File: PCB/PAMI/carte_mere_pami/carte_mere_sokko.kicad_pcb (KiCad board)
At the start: 2 copper layers, 78.5 x 54 mm, 35 parts, among them IC1 ESP32-S3-WROOM-1-N16R8, IC2 LDO_3.3V_bis, J1 Conn_01x08_Socket, J10 Conn_01x07_Socket, J11 Conn_01x07_Socket, J12 Conn_Servos, J14 LiDAR Connector, J2 Connector 5V, J3 Connector 3.3V, J4 Micro_USB_pads_USB3075-30-A, J5 Conn_01x08_Socket, J6 Conn_01x04_Pin, J7 Conn_01x04_Pin, J8 Conn_01x08_Socket, J9 Conn_01x08_Socket, U1 ICM-45686

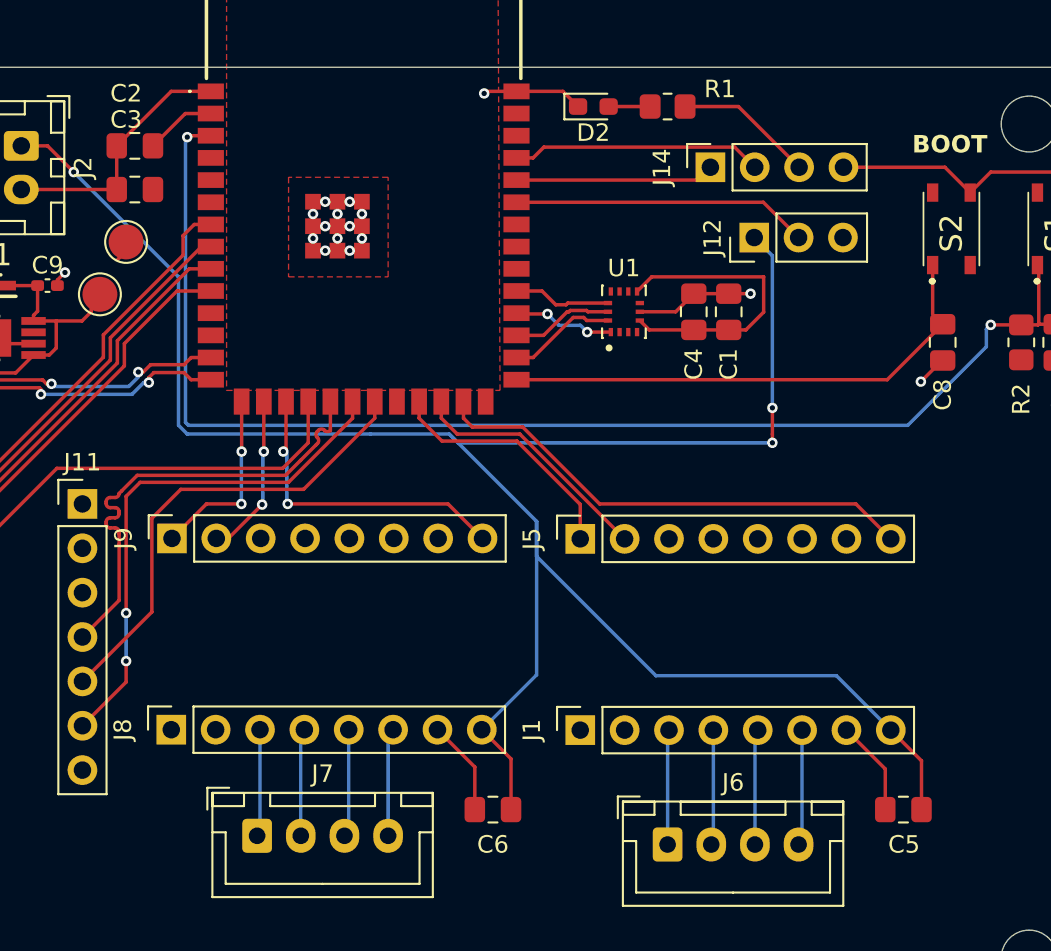
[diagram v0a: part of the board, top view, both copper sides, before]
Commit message: Update hole position
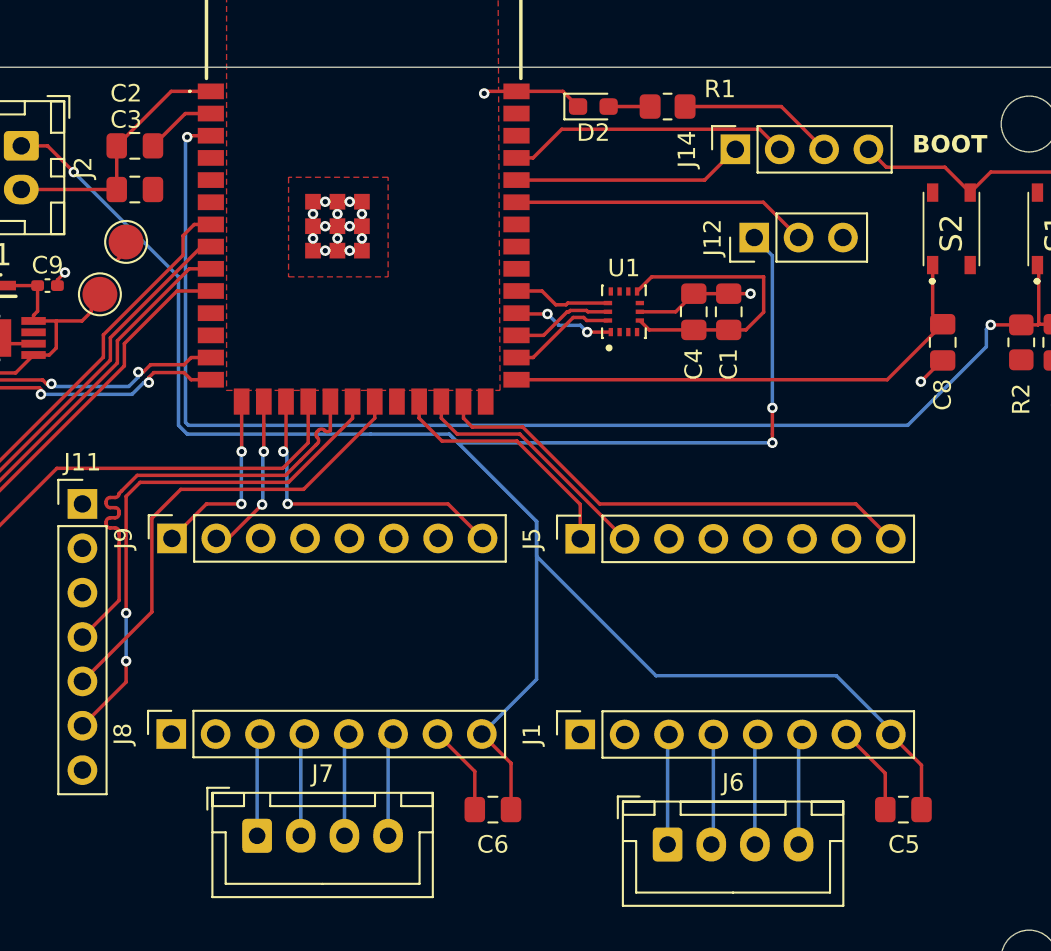
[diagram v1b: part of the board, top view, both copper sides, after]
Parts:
- moved J14 1.76 mm to (184.9, 72.7)
- moved J1 0.25 mm to (176.0, 106.2)
- moved J8 0.25 mm to (152.6, 106.2)
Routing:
- net TX_LiDAR: track 11.4 -> 13.3 mm
- net RX_LiDAR: track 14.4 -> 16.2 mm
- net GND: track 92.7 -> 91.2 mm
- net +3.3V: track 37.7 -> 38.7 mm
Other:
- board text added: "M1A"
- board text added: "M1B"
- board text added: "M2A"
- board text added: "M2B"
